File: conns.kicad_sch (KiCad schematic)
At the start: 3 parts, among them J31 Conn_01x20, J32 Conn_01x20, J33 Conn_01x20

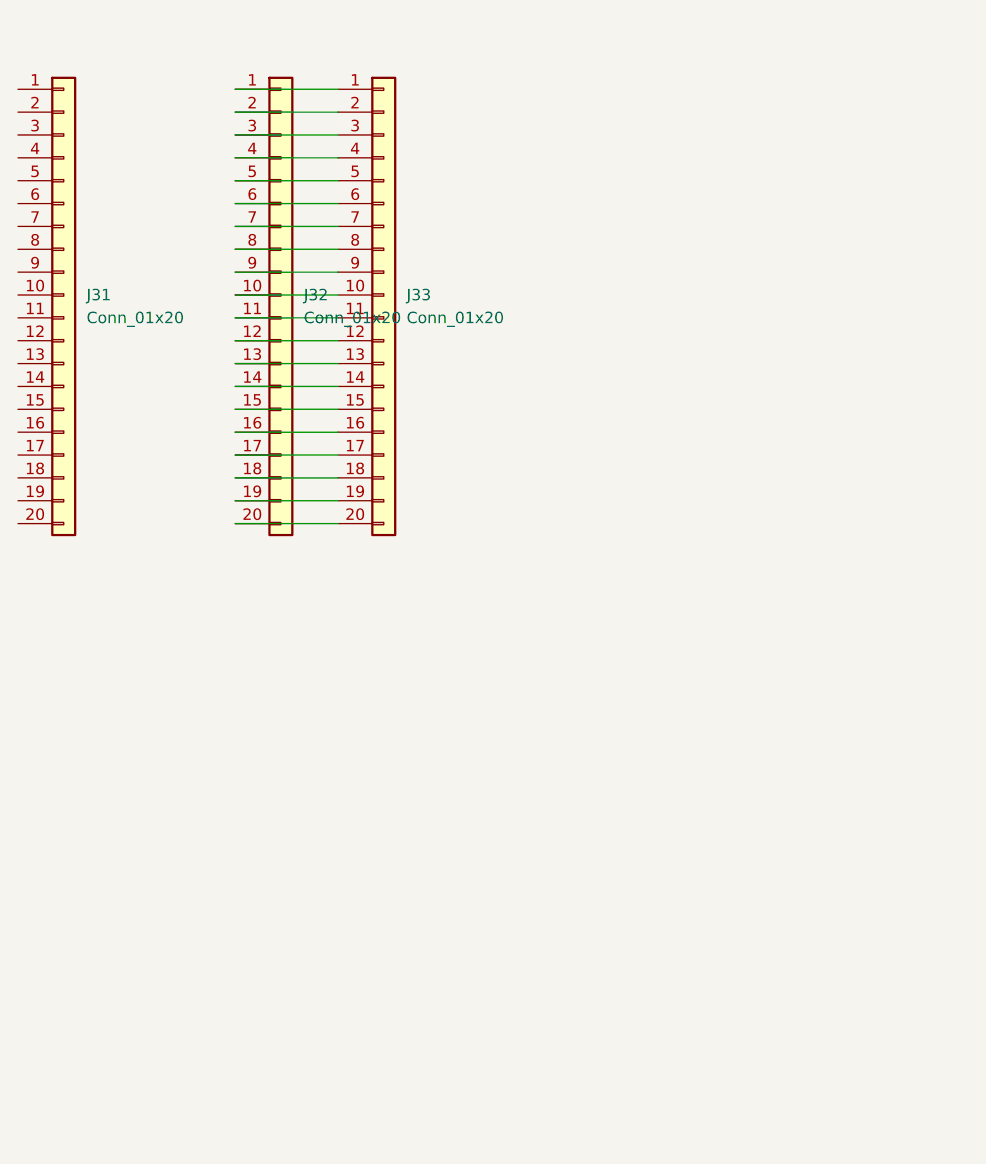
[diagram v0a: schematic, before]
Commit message: 更新
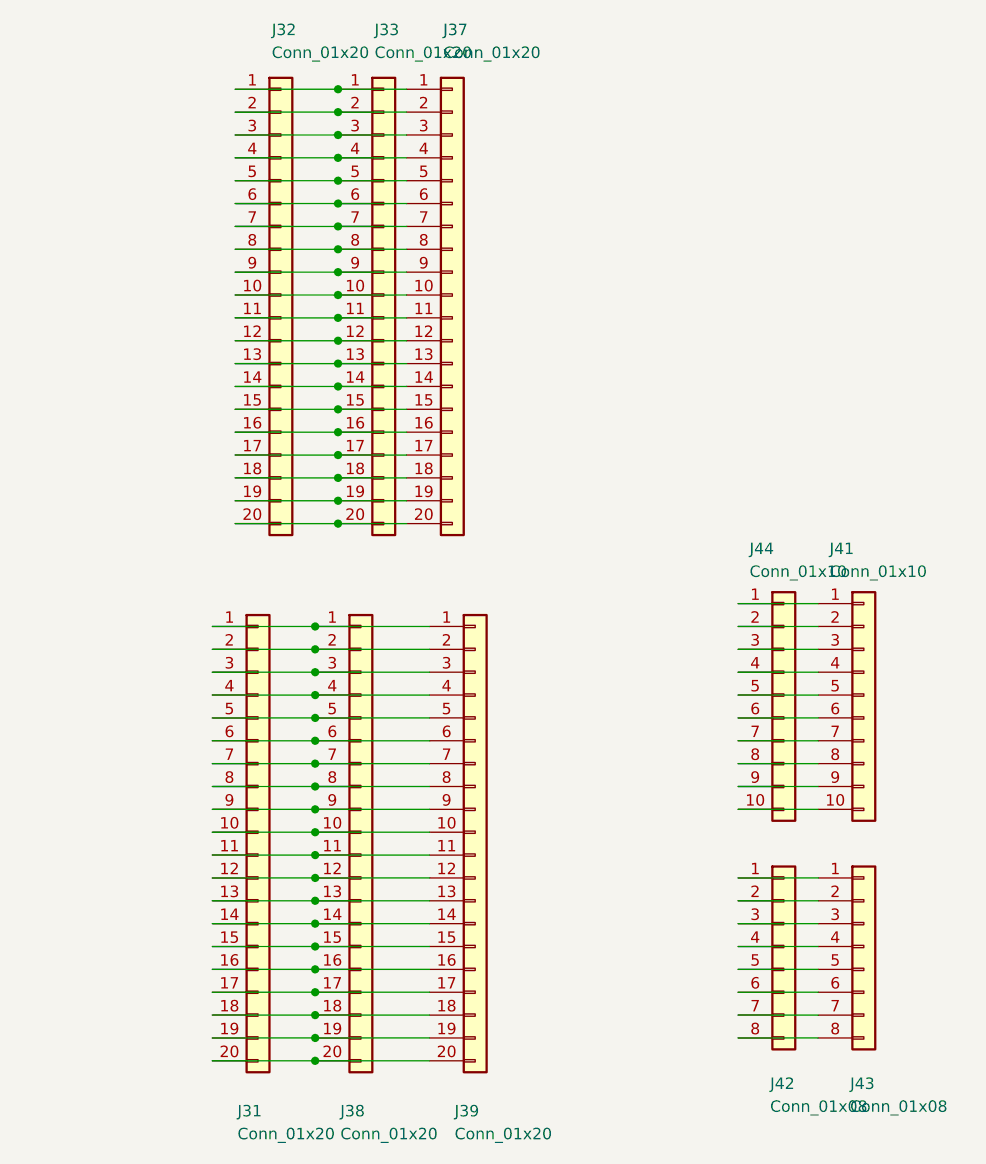
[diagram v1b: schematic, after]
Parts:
- added J37, J38, J39: Conn_01x20, Connector_PinSocket_2.54mm:PinSocket_1x20_P2.54mm_Vertical, symbol Connector_Generic:Conn_01x20
- added J41, J44: Conn_01x10, Connector_PinSocket_2.54mm:PinSocket_1x10_P2.54mm_Vertical, symbol Connector_Generic:Conn_01x10
- added J42, J43: Conn_01x08, Connector_PinSocket_2.54mm:PinSocket_1x08_P2.54mm_Vertical, symbol Connector_Generic:Conn_01x08
- J31, J32, J33: now left out of the parts list
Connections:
- net at J32.1 (Pin_1), J33.1 (Pin_1): now also J37.1 (Pin_1)
- net at J32.10 (Pin_10), J33.10 (Pin_10): now also J37.10 (Pin_10)
- net at J32.11 (Pin_11), J33.11 (Pin_11): now also J37.11 (Pin_11)
- net at J32.12 (Pin_12), J33.12 (Pin_12): now also J37.12 (Pin_12)
- net at J32.13 (Pin_13), J33.13 (Pin_13): now also J37.13 (Pin_13)
- net at J32.14 (Pin_14), J33.14 (Pin_14): now also J37.14 (Pin_14)
- net at J32.15 (Pin_15), J33.15 (Pin_15): now also J37.15 (Pin_15)
- net at J32.16 (Pin_16), J33.16 (Pin_16): now also J37.16 (Pin_16)
- net at J32.17 (Pin_17), J33.17 (Pin_17): now also J37.17 (Pin_17)
- net at J32.18 (Pin_18), J33.18 (Pin_18): now also J37.18 (Pin_18)
- net at J32.19 (Pin_19), J33.19 (Pin_19): now also J37.19 (Pin_19)
- net at J32.2 (Pin_2), J33.2 (Pin_2): now also J37.2 (Pin_2)
- net at J32.20 (Pin_20), J33.20 (Pin_20): now also J37.20 (Pin_20)
- net at J32.3 (Pin_3), J33.3 (Pin_3): now also J37.3 (Pin_3)
- net at J32.4 (Pin_4), J33.4 (Pin_4): now also J37.4 (Pin_4)
- net at J32.5 (Pin_5), J33.5 (Pin_5): now also J37.5 (Pin_5)
- net at J32.6 (Pin_6), J33.6 (Pin_6): now also J37.6 (Pin_6)
- net at J32.7 (Pin_7), J33.7 (Pin_7): now also J37.7 (Pin_7)
- net at J32.8 (Pin_8), J33.8 (Pin_8): now also J37.8 (Pin_8)
- net at J32.9 (Pin_9), J33.9 (Pin_9): now also J37.9 (Pin_9)
- net at J31.1 (Pin_1): now also J38.1 (Pin_1), J39.1 (Pin_1)
- net at J31.10 (Pin_10): now also J38.10 (Pin_10), J39.10 (Pin_10)
- net at J31.11 (Pin_11): now also J38.11 (Pin_11), J39.11 (Pin_11)
- net at J31.12 (Pin_12): now also J38.12 (Pin_12), J39.12 (Pin_12)
- net at J31.13 (Pin_13): now also J38.13 (Pin_13), J39.13 (Pin_13)
- net at J31.14 (Pin_14): now also J38.14 (Pin_14), J39.14 (Pin_14)
- net at J31.15 (Pin_15): now also J38.15 (Pin_15), J39.15 (Pin_15)
- net at J31.16 (Pin_16): now also J38.16 (Pin_16), J39.16 (Pin_16)
- net at J31.17 (Pin_17): now also J38.17 (Pin_17), J39.17 (Pin_17)
- net at J31.18 (Pin_18): now also J38.18 (Pin_18), J39.18 (Pin_18)
- net at J31.19 (Pin_19): now also J38.19 (Pin_19), J39.19 (Pin_19)
- net at J31.2 (Pin_2): now also J38.2 (Pin_2), J39.2 (Pin_2)
- net at J31.20 (Pin_20): now also J38.20 (Pin_20), J39.20 (Pin_20)
- net at J31.3 (Pin_3): now also J38.3 (Pin_3), J39.3 (Pin_3)
- net at J31.4 (Pin_4): now also J38.4 (Pin_4), J39.4 (Pin_4)
- net at J31.5 (Pin_5): now also J38.5 (Pin_5), J39.5 (Pin_5)
- net at J31.6 (Pin_6): now also J38.6 (Pin_6), J39.6 (Pin_6)
- net at J31.7 (Pin_7): now also J38.7 (Pin_7), J39.7 (Pin_7)
- net at J31.8 (Pin_8): now also J38.8 (Pin_8), J39.8 (Pin_8)
- net at J31.9 (Pin_9): now also J38.9 (Pin_9), J39.9 (Pin_9)
- new net: J42.1 (Pin_1), J43.1 (Pin_1)
- new net: J42.2 (Pin_2), J43.2 (Pin_2)
- new net: J42.3 (Pin_3), J43.3 (Pin_3)
- new net: J42.4 (Pin_4), J43.4 (Pin_4)
- new net: J42.5 (Pin_5), J43.5 (Pin_5)
- new net: J42.6 (Pin_6), J43.6 (Pin_6)
- new net: J42.7 (Pin_7), J43.7 (Pin_7)
- new net: J42.8 (Pin_8), J43.8 (Pin_8)
- new net: J41.1 (Pin_1), J44.1 (Pin_1)
- new net: J41.10 (Pin_10), J44.10 (Pin_10)
- new net: J41.2 (Pin_2), J44.2 (Pin_2)
- new net: J41.3 (Pin_3), J44.3 (Pin_3)
- new net: J41.4 (Pin_4), J44.4 (Pin_4)
- new net: J41.5 (Pin_5), J44.5 (Pin_5)
- new net: J41.6 (Pin_6), J44.6 (Pin_6)
- new net: J41.7 (Pin_7), J44.7 (Pin_7)
- new net: J41.8 (Pin_8), J44.8 (Pin_8)
- new net: J41.9 (Pin_9), J44.9 (Pin_9)
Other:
- moved on the sheet: J31
